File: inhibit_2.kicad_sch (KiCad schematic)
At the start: 3 parts, among them SW3 SAFE_switch

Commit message: Updated files and include work done for PCB
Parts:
- R7, R9: footprint (none) -> Resistor_SMD:R_0201_0603Metric
- SW3: footprint (none) -> Connector_PinHeader_2.54mm:PinHeader_1x02_P2.54mm_Vertical
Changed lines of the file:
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@@
 			)
 		)
-		(property "Footprint" ""
+		(property "Footprint" "Resistor_SMD:R_0201_0603Metric"
 			(at 54.356 54.356 90)
 			(effects
@@
 			)
 		)
-		(property "Footprint" ""
+		(property "Footprint" "Resistor_SMD:R_0201_0603Metric"
 			(at 40.386 54.356 90)
 			(effects
@@
 			)
 		)
-		(property "Footprint" ""
+		(property "Footprint" "Connector_PinHeader_2.54mm:PinHeader_1x02_P2.54mm_Vertical"
 			(at 54.61 67.31 0)
 			(effects

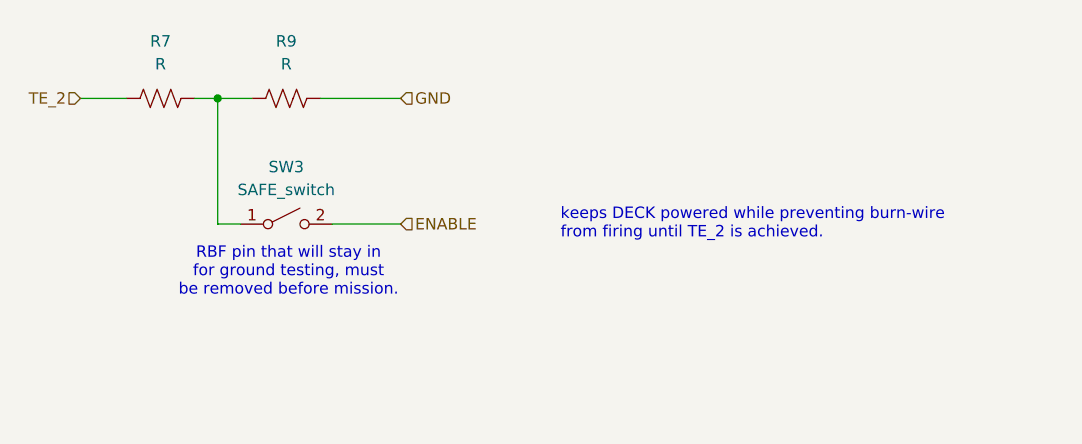
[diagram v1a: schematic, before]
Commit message: PCB is mostly laid out, routing is WIP
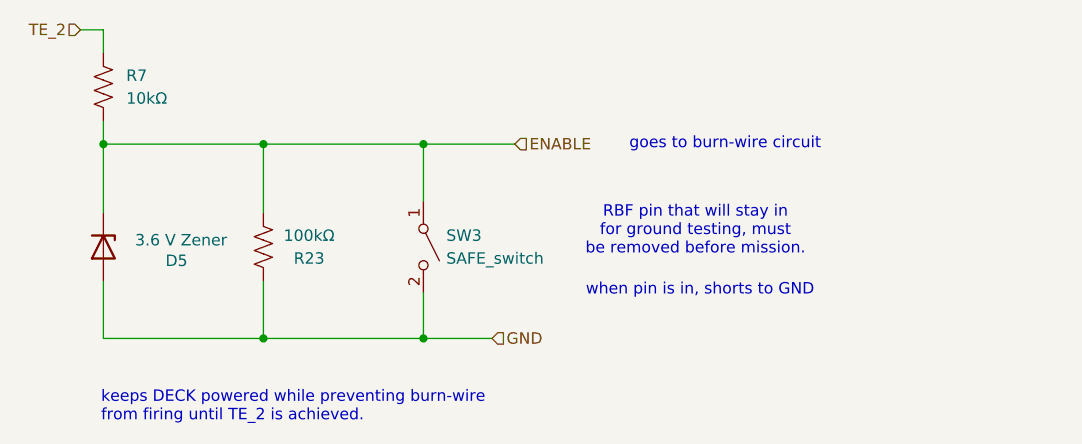
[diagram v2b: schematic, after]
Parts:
- removed R9: R, Resistor_SMD:R_0201_0603Metric, symbol Device:R_US
- added D5: 3.6 V Zener, Diode_SMD:D_SOD-123, symbol Device:D_Zener
- added R23: 100kΩ, Resistor_SMD:R_0201_0603Metric, symbol Device:R_US
- R7: value R -> 10kΩ
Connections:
- net ENABLE: now also R7.1, SW3.1 (A), D5.1 (K), R23.1; no longer SW3.2 (B)
- net GND: now also SW3.2 (B), D5.2 (A), R23.2
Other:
- note added: "goes to burn-wire circuit"
- note added: "when pin is in, shorts to GND"
- moved on the sheet: R7, SW3

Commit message: Finished PCB, ready to print
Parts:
- SW3: footprint Connector_PinHeader_2.54mm:PinHeader_1x02_P2.54mm_Vertical -> Connector_PinHeader_2.54mm:PinHeader_1x01_P2.54mm_Vertical
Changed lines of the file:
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@@
 			)
 		)
-		(property "Footprint" "Connector_PinHeader_2.54mm:PinHeader_1x02_P2.54mm_Vertical"
+		(property "Footprint" "Connector_PinHeader_2.54mm:PinHeader_1x01_P2.54mm_Vertical"
 			(at 69.85 69.85 0)
 			(effects
